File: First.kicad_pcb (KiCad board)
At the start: 2 copper layers, 54.1 x 51.8 mm, 48 parts, among them J1 UART0, J2 UART1, J3 USB_B_Micro, J4 UART2, J5 UART3, U1 CP2102N-DEV0, U2 TUSB2046IBVFR, U3 CP2102N-DEV1, U4 CP2102N_DEV2, U5 LD1086V33-DG, U6 CP2102N-A01-GQFN24, Y1 HC49SDLF-8.00MHz

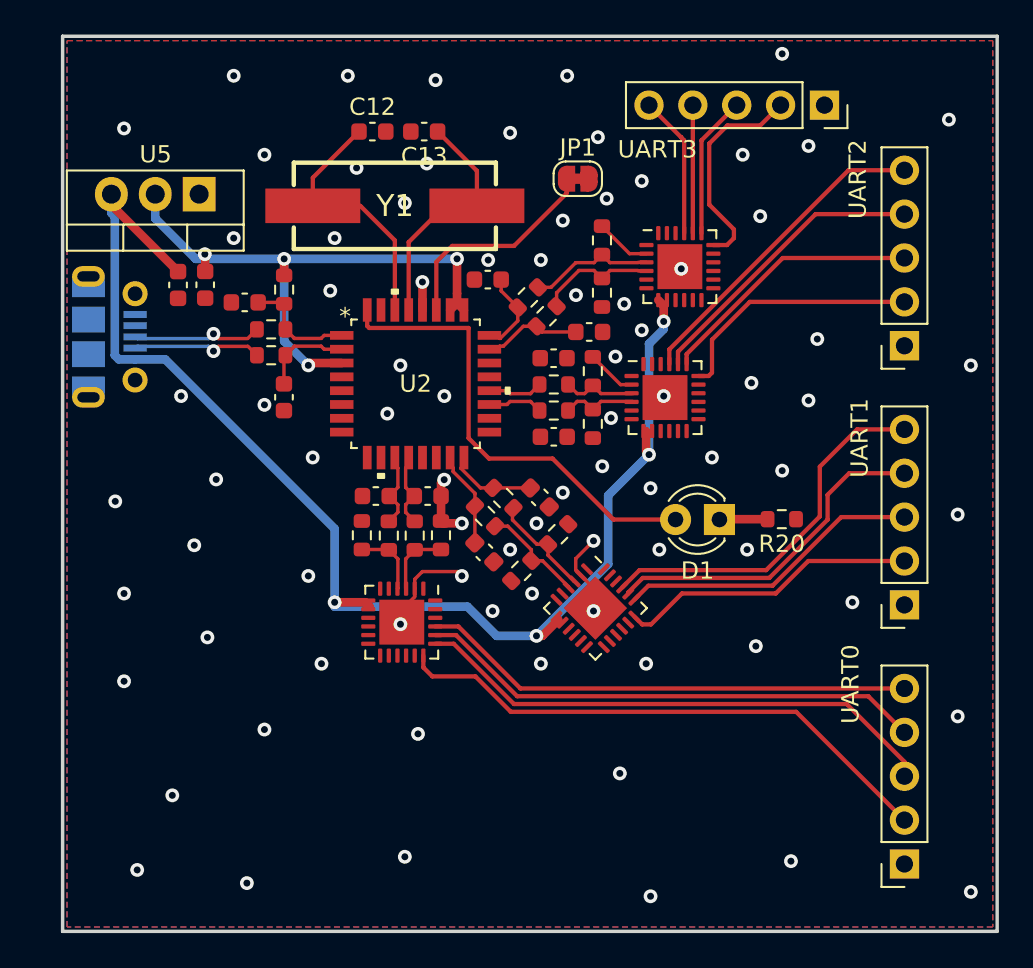
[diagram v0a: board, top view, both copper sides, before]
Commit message: Ordered version
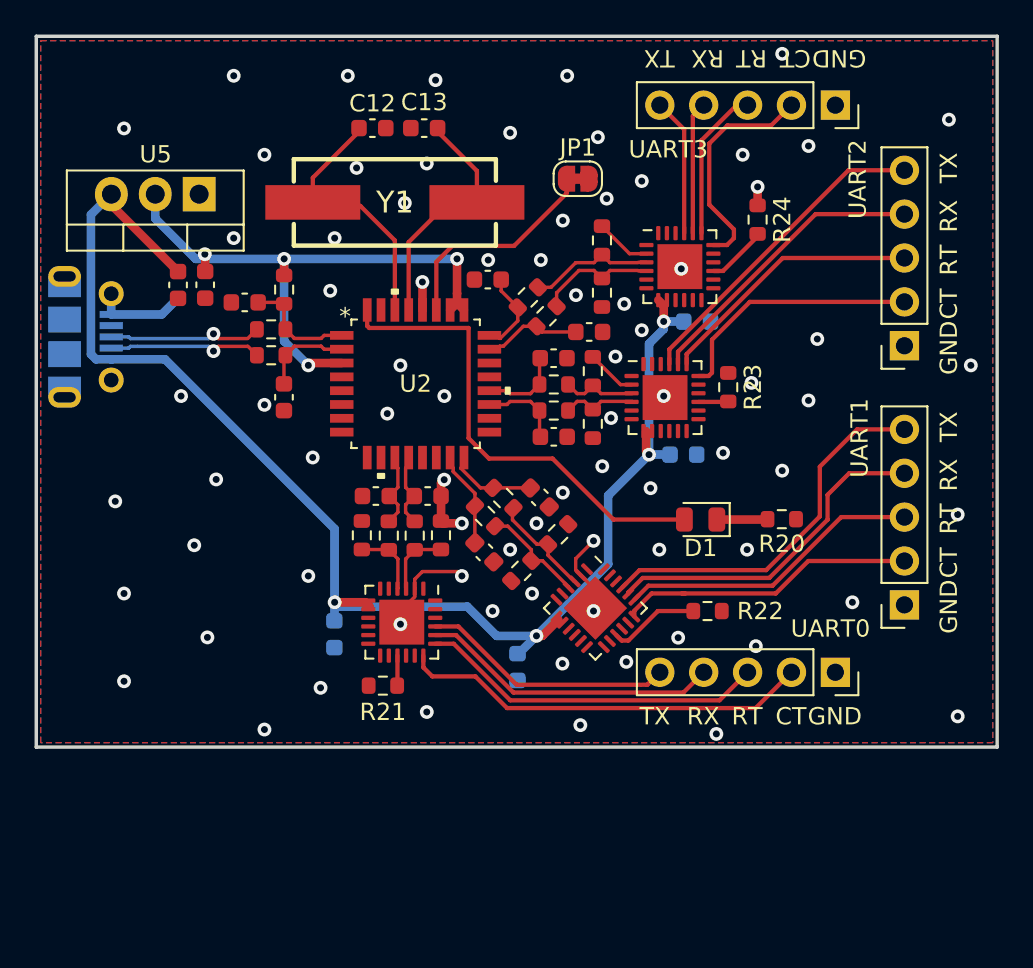
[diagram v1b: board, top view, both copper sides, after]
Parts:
- added C14: 22p, Capacitor_SMD:C_0603_1608Metric, B.Cu at (132.2, 61.3)
- added C15: 22p, Capacitor_SMD:C_0603_1608Metric, B.Cu at (122.6, 73.6)
- added C16: 22p, Capacitor_SMD:C_0603_1608Metric, B.Cu at (133.0, 53.6)
- added C17: 22p, Capacitor_SMD:C_0603_1608Metric, B.Cu at (112.0, 71.7)
- added G***: LOGO, LOGO, B.Cu at (116.0, 63.8)
- added R21: 10k, Resistor_SMD:R_0603_1608Metric, F.Cu at (114.8, 74.7)
- added R22: 10k, Resistor_SMD:R_0603_1608Metric, F.Cu at (133.6, 70.4)
- added R23: 10k, Resistor_SMD:R_0603_1608Metric, F.Cu at (134.8, 57.4)
- added R24: 10k, Resistor_SMD:R_0603_1608Metric, F.Cu at (136.5, 47.7)
- D1: footprint LED_THT:LED_D3.0mm -> LED_SMD:LED_0805_2012Metric
- moved J1 11.8 mm to (141.0, 73.9), turned to -90 degrees
- moved J3 1.38 mm to (97.6, 54.5)
- moved D1 1.09 mm to (133.2, 65.1)
- moved J5 0.63 mm to (141.0, 41.1)
- moved C12 0.20 mm to (114.2, 42.4)
- moved C13 0.20 mm to (117.2, 42.4)
- moved Y1 0.20 mm to (115.5, 46.7)
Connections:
- U1 pad 15: unconnected-(U1-Pad15) -> Net-(U1-Pad15)
- U3 pad 15: unconnected-(U3-Pad15) -> Net-(U3-Pad15)
- U4 pad 15: unconnected-(U4-Pad15) -> Net-(U4-Pad15)
- U6 pad 15: unconnected-(U6-Pad15) -> Net-(U6-Pad15)
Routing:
- net /TX_0: track 28.6 -> 14.6 mm
- net /RX_0: track 29.5 -> 17.4 mm
- net /RTS_0: track 30.8 -> 20.1 mm
- net /CTS_0: track 32.2 -> 23.8 mm
- net VBUS: track 77.5 -> 84.2 mm
- net GND: track 22.2 -> 28.6 mm, vias 83 -> 78
- net Net-(U3-Pad15): track 0.00 -> 5.31 mm
- net Net-(U6-Pad15): track 0.00 -> 3.53 mm
- net Net-(U4-Pad15): track 0.00 -> 1.73 mm
- net Net-(U1-Pad15): track 0.00 -> 1.66 mm
- net /D-2: track 3.22 -> 4.76 mm
- net /D+2: track 3.22 -> 4.76 mm
- net /USB_IN+: track 7.50 -> 8.86 mm
- net /USB_IN-: track 7.50 -> 8.86 mm
- net /CTS_3: track 12.5 -> 13.1 mm
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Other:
- board size 54.1 x 51.8 mm -> 55.6 x 41.1 mm
- board text added: "CT"
- board text added: "GND"
- board text added: "RT"
- board text added: "RX"
- board text added: "TX"
